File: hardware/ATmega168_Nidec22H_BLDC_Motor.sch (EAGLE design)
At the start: 17 parts, among them IC2 ATMEGA168-20P, X1 14.7456 MHz

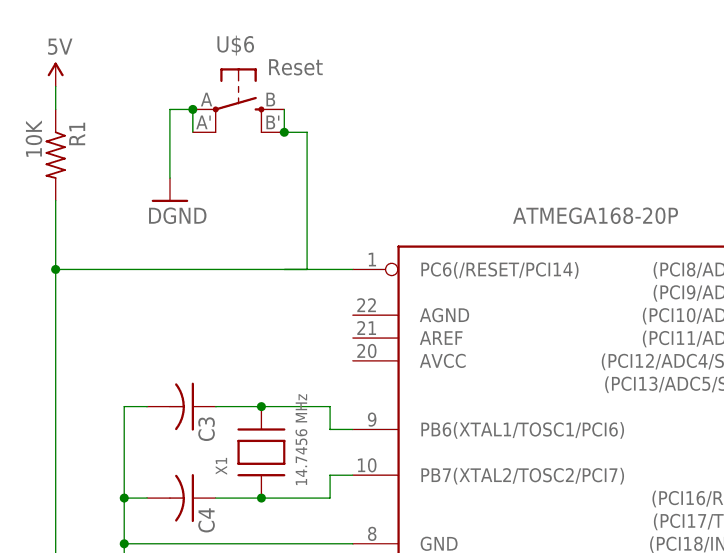
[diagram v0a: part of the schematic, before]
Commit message: Labeled nets
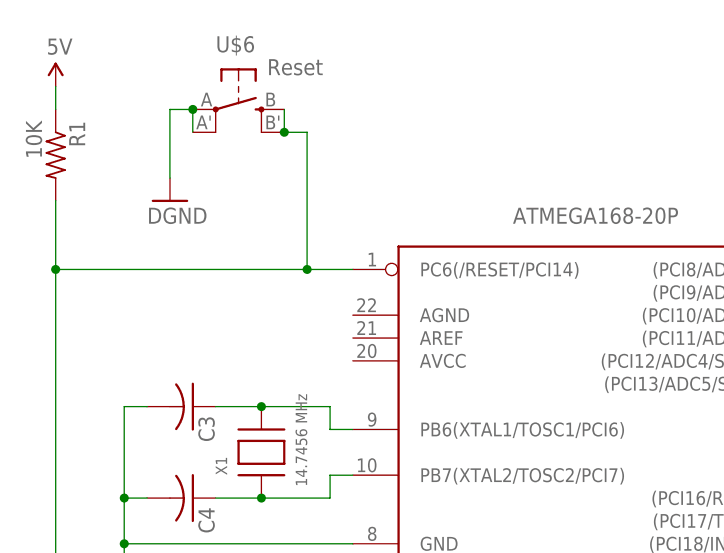
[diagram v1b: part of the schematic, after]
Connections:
- net N$10 renamed TXD
- net N$11 renamed RXD
- net N$12 renamed 24V
- net N$14 renamed DIR-1
- net N$15 renamed TACH-1
- net N$17 renamed PWM-1
- net N$18 renamed EN-1
- net N$19 renamed DIR-2
- net N$21 renamed PWM-2
- net N$22 renamed EN-2
- net N$5 renamed SCK
- net N$6 renamed MISO
- net N$7 renamed MOSI
- net SS&REQ renamed TACH-2
- removed net N$16: IC2.PC6(/RESET/PCI14)
- removed net N$8: ISP1.RST, R1.2, U$6.S, U$6.S1
- removed net N$9: ISP1.VCC
- new net RST: IC2.PC6(/RESET/PCI14), ISP1.RST, R1.2, U$6.S, U$6.S1
- net 5V: now also ISP1.VCC
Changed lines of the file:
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@@
 <setting verticaltext="up"/>
 </settings>
-<grid distance="0.1" unitdist="inch" unit="inch" style="lines" multiple="1" display="no" altdistance="0.01" altunitdist="inch" altunit="inch"/>
+<grid distance="0.05" unitdist="inch" unit="inch" style="lines" multiple="1" display="yes" altdistance="0.01" altunitdist="inch" altunit="inch"/>
 <layers>
 <layer number="1" name="Top" color="4" fill="1" visible="no" active="no"/>
@@
 <junction x="160.02" y="64.77"/>
 </segment>
+<segment>
+<pinref part="ISP1" gate="G$1" pin="VCC"/>
+<wire x1="101.6" y1="52.07" x2="104.14" y2="52.07" width="0.1524" layer="91"/>
+</segment>
 </net>
 <net name="N$3" class="0">
@@
 </segment>
 </net>
-<net name="N$5" class="0">
+<net name="SCK" class="0">
 <segment>
 <pinref part="IC2" gate="G$1" pin="(PCI5/SCK)PB5"/>
@@
 </segment>
 </net>
-<net name="N$6" class="0">
+<net name="MISO" class="0">
 <segment>
 <pinref part="IC2" gate="G$1" pin="(PCI4/MISO)PB4"/>
@@
 </segment>
 </net>
-<net name="N$7" class="0">
+<net name="MOSI" class="0">
 <segment>
 <pinref part="IC2" gate="G$1" pin="(PCI3/MOSI/OC2A)PB3"/>
@@
 </segment>
 </net>
-<net name="N$9" class="0">
-<segment>
-<pinref part="ISP1" gate="G$1" pin="VCC"/>
-<wire x1="101.6" y1="52.07" x2="104.14" y2="52.07" width="0.1524" layer="91"/>
-</segment>
-</net>
-<net name="SS&amp;REQ" class="0">
+<net name="TACH-2" class="0">
 <segment>
 <pinref part="IC2" gate="G$1" pin="(PCI1/OC1A/OC1S)PB1"/>
@@
 </segment>
 </net>
-<net name="N$10" class="0">
+<net name="TXD" class="0">
 <segment>
 <pinref part="IC2" gate="G$1" pin="(PCI16/RXD)PD0"/>
@@
 </segment>
 </net>
-<net name="N$11" class="0">
+<net name="RXD" class="0">
 <segment>
 <pinref part="IC2" gate="G$1" pin="(PCI17/TXD)PD1"/>
@@
 </segment>
 </net>
-<net name="N$12" class="0">
+<net name="24V" class="0">
 <segment>
 <pinref part="12V" gate="G$1" pin="TIP"/>
@@
 </segment>
 </net>
-<net name="N$14" class="0">
+<net name="DIR-1" class="0">
 <segment>
 <pinref part="IC2" gate="G$1" pin="(PCI8/ADC0)PC0"/>
@@
 </segment>
 </net>
-<net name="N$15" class="0">
+<net name="TACH-1" class="0">
 <segment>
 <pinref part="JP3" gate="A" pin="4"/>
@@
 </segment>
 </net>
-<net name="N$17" class="0">
+<net name="PWM-1" class="0">
 <segment>
 <wire x1="157.48" y1="97.79" x2="157.48" y2="135.89" width="0.1524" layer="91"/>
@@
 </segment>
 </net>
-<net name="N$18" class="0">
+<net name="EN-1" class="0">
 <segment>
 <pinref part="IC2" gate="G$1" pin="(PCI10/ADC2)PC2"/>
@@
 </segment>
 </net>
-<net name="N$19" class="0">
+<net name="DIR-2" class="0">
 <segment>
 <pinref part="IC2" gate="G$1" pin="(PCI9/ADC1)PC1"/>
@@
 </segment>
 </net>
-<net name="N$21" class="0">
+<net name="PWM-2" class="0">
 <segment>
 <pinref part="JP4" gate="A" pin="5"/>
@@
 </segment>
 </net>
-<net name="N$22" class="0">
+<net name="EN-2" class="0">
 <segment>
 <pinref part="IC2" gate="G$1" pin="(PCI11/ADC3)PC3"/>
@@
 </segment>
 </net>
-<net name="N$8" class="0">
+<net name="N$1" class="0">
+<segment>
+<pinref part="IC2" gate="G$1" pin="(PCI2/SS/OC1B)PB2"/>
+<pinref part="R2" gate="G$1" pin="1"/>
+<wire x1="114.3" y1="85.09" x2="134.62" y2="85.09" width="0.1524" layer="91"/>
+</segment>
+</net>
+<net name="N$13" class="0">
+<segment>
+<pinref part="R2" gate="G$1" pin="2"/>
+<pinref part="LED1" gate="G$1" pin="A"/>
+</segment>
+</net>
+<net name="RST" class="0">
 <segment>
 <pinref part="U$6" gate="G$1" pin="S"/>
@@
 <junction x="50.8" y="153.67"/>
 <pinref part="ISP1" gate="G$1" pin="RST"/>
-<wire x1="53.34" y1="138.43" x2="25.4" y2="138.43" width="0.1524" layer="91"/>
 <wire x1="73.66" y1="46.99" x2="25.4" y2="46.99" width="0.1524" layer="91"/>
 <wire x1="25.4" y1="46.99" x2="25.4" y2="138.43" width="0.1524" layer="91"/>
 <pinref part="R1" gate="G$1" pin="2"/>
+<pinref part="IC2" gate="G$1" pin="PC6(/RESET/PCI14)"/>
 <wire x1="25.4" y1="138.43" x2="25.4" y2="146.05" width="0.1524" layer="91"/>
+<wire x1="58.42" y1="138.43" x2="53.34" y2="138.43" width="0.1524" layer="91"/>
 <junction x="25.4" y="138.43"/>
+<wire x1="53.34" y1="138.43" x2="25.4" y2="138.43" width="0.1524" layer="91"/>
 <wire x1="53.34" y1="153.67" x2="53.34" y2="138.43" width="0.1524" layer="91"/>
-</segment>
-</net>
-<net name="N$16" class="0">
-<segment>
-<pinref part="IC2" gate="G$1" pin="PC6(/RESET/PCI14)"/>
-<wire x1="58.42" y1="138.43" x2="50.8" y2="138.43" width="0.1524" layer="91"/>
-</segment>
-</net>
-<net name="N$1" class="0">
-<segment>
-<pinref part="IC2" gate="G$1" pin="(PCI2/SS/OC1B)PB2"/>
-<pinref part="R2" gate="G$1" pin="1"/>
-<wire x1="114.3" y1="85.09" x2="134.62" y2="85.09" width="0.1524" layer="91"/>
-</segment>
-</net>
-<net name="N$13" class="0">
-<segment>
-<pinref part="R2" gate="G$1" pin="2"/>
-<pinref part="LED1" gate="G$1" pin="A"/>
-</segment>
-</net>
+<junction x="53.34" y="138.43"/>
+</segment>
+</net>
